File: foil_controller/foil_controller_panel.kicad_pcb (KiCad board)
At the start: 2 copper layers, 90 x 110 mm, 4 parts

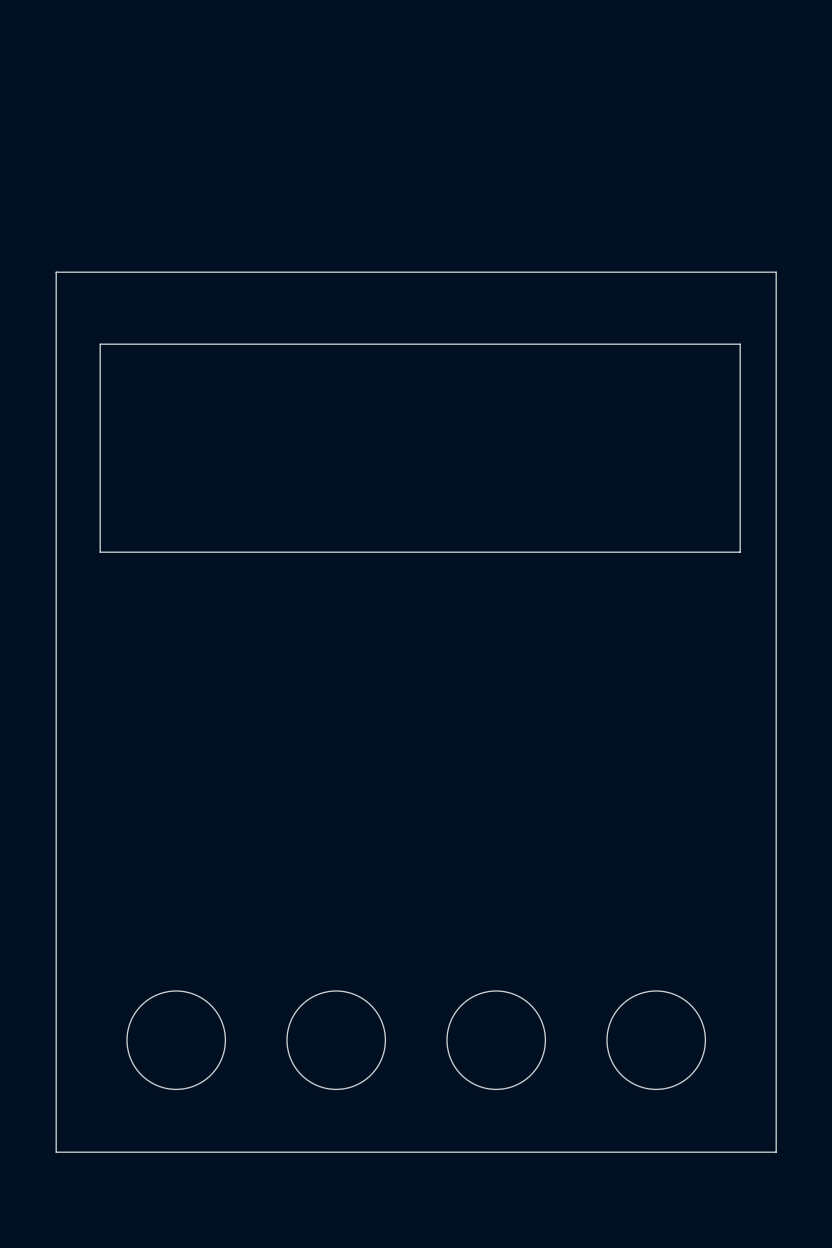
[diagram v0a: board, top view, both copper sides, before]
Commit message: controller v2 voor testvaart 1 mei
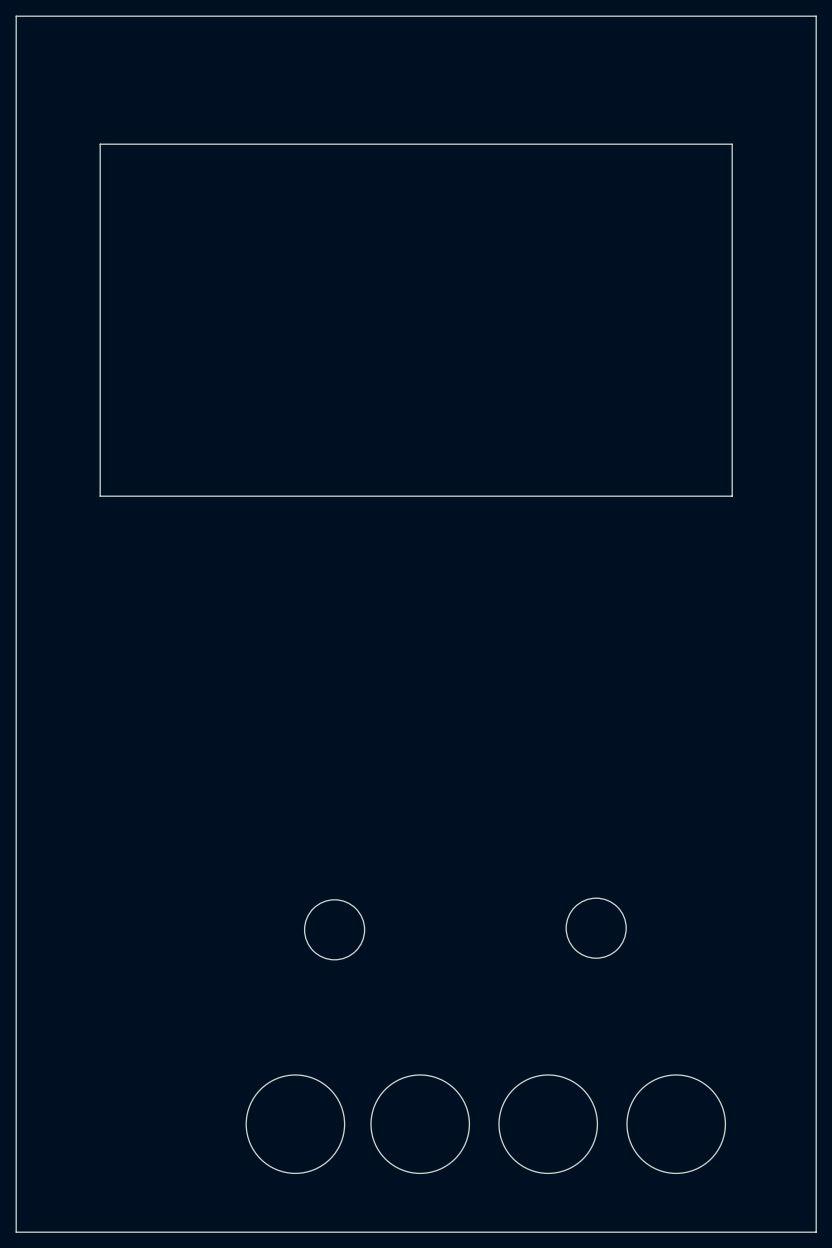
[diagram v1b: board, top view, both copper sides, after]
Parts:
- removed the H1 at (15.0, 96.0)
- removed the H1 at (35.0, 96.0)
- removed the H1 at (75.0, 96.0)
- removed the H1 at (55.0, 96.0)
- added H1: hole, MountingHole:MountingHole_3.2mm_M3_DIN965, F.Cu at (67.5, 82.0)
- added H1: hole, MountingHole:MountingHole_3.2mm_M3_DIN965, F.Cu at (34.8, 82.2)
- added H1: hole, MountingHole:MountingHole_3.2mm_M3_DIN965, F.Cu at (29.9, 106.5)
- added H1: hole, MountingHole:MountingHole_3.2mm_M3_DIN965, F.Cu at (45.5, 106.5)
- added H1: hole, MountingHole:MountingHole_3.2mm_M3_DIN965, F.Cu at (77.5, 106.5)
- added H1: hole, MountingHole:MountingHole_3.2mm_M3_DIN965, F.Cu at (61.5, 106.5)
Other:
- board size 90 x 110 mm -> 100 x 152 mm
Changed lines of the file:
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@@
     (tracks 0)
     (zones 0)
-    (modules 4)
+    (modules 6)
     (nets 1)
   )
@@
       (outputformat 1)
       (mirror false)
-      (drillshape 0)
+      (drillshape 1)
       (scaleselection 1)
-      (outputdirectory "out/"))
+      (outputdirectory ""))
   )
   (net 0 "")
@@
   )
   (module MountingHole:MountingHole_3.2mm_M3_DIN965 (layer F.Cu)
-    (at 15 96)
-    (descr hole)
-    (tags hole)
-    (attr virtual)
-    (fp_text reference H1 (at 0 -3.8) (layer F.SilkS) hide
-      (effects (font (size 1 1) (thickness 0.15)))
-    )
-    (fp_text value hole (at 0 3.8) (layer F.Fab) hide
-      (effects (font (size 1 1) (thickness 0.15)))
-    )
-    (fp_circle (center 0 0) (end 3.05 0) (layer F.CrtYd) (width 0.05))
-    (fp_circle (center 0 0) (end 2.8 0) (layer Cmts.User) (width 0.15))
-    (fp_text user %R (at 0.3 0) (layer F.Fab)
-      (effects (font (size 1 1) (thickness 0.15)))
-    )
-    (pad 1 np_thru_hole circle (at 0 0) (size 12.3 12.3) (drill 12.3) (layers *.Cu *.Mask))
-  )
-  (module MountingHole:MountingHole_3.2mm_M3_DIN965 (layer F.Cu)
-    (at 35 96)
-    (descr hole)
-    (tags hole)
-    (attr virtual)
-    (fp_text reference H1 (at 0 -3.8) (layer F.SilkS) hide
-      (effects (font (size 1 1) (thickness 0.15)))
-    )
-    (fp_text value hole (at 0 3.8) (layer F.Fab) hide
-      (effects (font (size 1 1) (thickness 0.15)))
-    )
-    (fp_circle (center 0 0) (end 3.05 0) (layer F.CrtYd) (width 0.05))
-    (fp_circle (center 0 0) (end 2.8 0) (layer Cmts.User) (width 0.15))
-    (fp_text user %R (at 0.3 0) (layer F.Fab)
-      (effects (font (size 1 1) (thickness 0.15)))
-    )
-    (pad 1 np_thru_hole circle (at 0 0) (size 12.3 12.3) (drill 12.3) (layers *.Cu *.Mask))
-  )
-  (module MountingHole:MountingHole_3.2mm_M3_DIN965 (layer F.Cu)
-    (at 75 96)
-    (descr hole)
-    (tags hole)
-    (attr virtual)
-    (fp_text reference H1 (at 0 -3.8) (layer F.SilkS) hide
-      (effects (font (size 1 1) (thickness 0.15)))
-    )
-    (fp_text value hole (at 0 3.8) (layer F.Fab) hide
-      (effects (font (size 1 1) (thickness 0.15)))
-    )
-    (fp_circle (center 0 0) (end 3.05 0) (layer F.CrtYd) (width 0.05))
-    (fp_circle (center 0 0) (end 2.8 0) (layer Cmts.User) (width 0.15))
-    (fp_text user %R (at 0.3 0) (layer F.Fab)
-      (effects (font (size 1 1) (thickness 0.15)))
-    )
-    (pad 1 np_thru_hole circle (at 0 0) (size 12.3 12.3) (drill 12.3) (layers *.Cu *.Mask))
-  )
-  (module MountingHole:MountingHole_3.2mm_M3_DIN965 (layer F.Cu)
-    (at 55 96)
-    (descr hole)
-    (tags hole)
-    (attr virtual)
-    (fp_text reference H1 (at 0 -3.8) (layer F.SilkS) hide
-      (effects (font (size 1 1) (thickness 0.15)))
-    )
-    (fp_text value hole (at 0 3.8) (layer F.Fab) hide
-      (effects (font (size 1 1) (thickness 0.15)))
-    )
-    (fp_circle (center 0 0) (end 3.05 0) (layer F.CrtYd) (width 0.05))
-    (fp_circle (center 0 0) (end 2.8 0) (layer Cmts.User) (width 0.15))
-    (fp_text user %R (at 0.3 0) (layer F.Fab)
-      (effects (font (size 1 1) (thickness 0.15)))
-    )
-    (pad 1 np_thru_hole circle (at 0 0) (size 12.3 12.3) (drill 12.3) (layers *.Cu *.Mask))
-  )
-  (gr_line (start 5.5 35) (end 85.5 35) (layer Edge.Cuts) (width 0.05))
-  (gr_line (start 5.5 9) (end 5.5 35) (layer Edge.Cuts) (width 0.05))
-  (gr_line (start 85.5 9) (end 5.5 9) (layer Edge.Cuts) (width 0.05))
-  (gr_line (start 85.5 35) (end 85.5 9) (layer Edge.Cuts) (width 0.05))
-  (gr_line (start 0 110) (end 0 0) (layer Edge.Cuts) (width 0.05))
-  (gr_line (start 90 110) (end 0 110) (layer Edge.Cuts) (width 0.05))
-  (gr_line (start 90 0) (end 90 110) (layer Edge.Cuts) (width 0.05))
-  (gr_line (start 0 0) (end 90 0) (layer Edge.Cuts) (width 0.05))
+    (at 67.5 82)
+    (descr hole)
+    (tags hole)
+    (attr virtual)
+    (fp_text reference H1 (at 0 -3.8) (layer F.SilkS) hide
+      (effects (font (size 1 1) (thickness 0.15)))
+    )
+    (fp_text value hole (at 0 3.8) (layer F.Fab) hide
+      (effects (font (size 1 1) (thickness 0.15)))
+    )
+    (fp_circle (center 0 0) (end 3.05 0) (layer F.CrtYd) (width 0.05))
+    (fp_circle (center 0 0) (end 2.8 0) (layer Cmts.User) (width 0.15))
+    (fp_text user %R (at 0.3 0) (layer F.Fab)
+      (effects (font (size 1 1) (thickness 0.15)))
+    )
+    (pad 1 np_thru_hole circle (at 0 0) (size 7.5 7.5) (drill 7.5) (layers *.Cu *.Mask))
+  )
+  (module MountingHole:MountingHole_3.2mm_M3_DIN965 (layer F.Cu)
+    (at 34.8 82.2)
+    (descr hole)
+    (tags hole)
+    (attr virtual)
+    (fp_text reference H1 (at 0 -3.8) (layer F.SilkS) hide
+      (effects (font (size 1 1) (thickness 0.15)))
+    )
+    (fp_text value hole (at 0 3.8) (layer F.Fab) hide
+      (effects (font (size 1 1) (thickness 0.15)))
+    )
+    (fp_circle (center 0 0) (end 3.05 0) (layer F.CrtYd) (width 0.05))
+    (fp_circle (center 0 0) (end 2.8 0) (layer Cmts.User) (width 0.15))
+    (fp_text user %R (at 0.3 0) (layer F.Fab)
+      (effects (font (size 1 1) (thickness 0.15)))
+    )
+    (pad 1 np_thru_hole circle (at 0 0) (size 7.5 7.5) (drill 7.5) (layers *.Cu *.Mask))
+  )
+  (module MountingHole:MountingHole_3.2mm_M3_DIN965 (layer F.Cu)
+    (at 29.9 106.5)
+    (descr hole)
+    (tags hole)
+    (attr virtual)
+    (fp_text reference H1 (at 0 -3.8) (layer F.SilkS) hide
+      (effects (font (size 1 1) (thickness 0.15)))
+    )
+    (fp_text value hole (at 0 3.8) (layer F.Fab) hide
+      (effects (font (size 1 1) (thickness 0.15)))
+    )
+    (fp_circle (center 0 0) (end 3.05 0) (layer F.CrtYd) (width 0.05))
+    (fp_circle (center 0 0) (end 2.8 0) (layer Cmts.User) (width 0.15))
+    (fp_text user %R (at 0.3 0) (layer F.Fab)
+      (effects (font (size 1 1) (thickness 0.15)))
+    )
+    (pad 1 np_thru_hole circle (at 0 0) (size 12.3 12.3) (drill 12.3) (layers *.Cu *.Mask))
+  )
+  (module MountingHole:MountingHole_3.2mm_M3_DIN965 (layer F.Cu)
+    (at 45.5 106.5)
+    (descr hole)
+    (tags hole)
+    (attr virtual)
+    (fp_text reference H1 (at 0 -3.8) (layer F.SilkS) hide
+      (effects (font (size 1 1) (thickness 0.15)))
+    )
+    (fp_text value hole (at 0 3.8) (layer F.Fab) hide
+      (effects (font (size 1 1) (thickness 0.15)))
+    )
+    (fp_circle (center 0 0) (end 3.05 0) (layer F.CrtYd) (width 0.05))
+    (fp_circle (center 0 0) (end 2.8 0) (layer Cmts.User) (width 0.15))
+    (fp_text user %R (at 0.3 0) (layer F.Fab)
+      (effects (font (size 1 1) (thickness 0.15)))
+    )
+    (pad 1 np_thru_hole circle (at 0 0) (size 12.3 12.3) (drill 12.3) (layers *.Cu *.Mask))
+  )
+  (module MountingHole:MountingHole_3.2mm_M3_DIN965 (layer F.Cu)
+    (at 77.5 106.5)
+    (descr hole)
+    (tags hole)
+    (attr virtual)
+    (fp_text reference H1 (at 0 -3.8) (layer F.SilkS) hide
+      (effects (font (size 1 1) (thickness 0.15)))
+    )
+    (fp_text value hole (at 0 3.8) (layer F.Fab) hide
+      (effects (font (size 1 1) (thickness 0.15)))
+    )
+    (fp_circle (center 0 0) (end 3.05 0) (layer F.CrtYd) (width 0.05))
+    (fp_circle (center 0 0) (end 2.8 0) (layer Cmts.User) (width 0.15))
+    (fp_text user %R (at 0.3 0) (layer F.Fab)
+      (effects (font (size 1 1) (thickness 0.15)))
+    )
+    (pad 1 np_thru_hole circle (at 0 0) (size 12.3 12.3) (drill 12.3) (layers *.Cu *.Mask))
+  )
+  (module MountingHole:MountingHole_3.2mm_M3_DIN965 (layer F.Cu)
+    (at 61.5 106.5)
+    (descr hole)
+    (tags hole)
+    (attr virtual)
+    (fp_text reference H1 (at 0 -3.8) (layer F.SilkS) hide
+      (effects (font (size 1 1) (thickness 0.15)))
+    )
+    (fp_text value hole (at 0 3.8) (layer F.Fab) hide
+      (effects (font (size 1 1) (thickness 0.15)))
+    )
+    (fp_circle (center 0 0) (end 3.05 0) (layer F.CrtYd) (width 0.05))
+    (fp_circle (center 0 0) (end 2.8 0) (layer Cmts.User) (width 0.15))
+    (fp_text user %R (at 0.3 0) (layer F.Fab)
+      (effects (font (size 1 1) (thickness 0.15)))
+    )
+    (pad 1 np_thru_hole circle (at 0 0) (size 12.3 12.3) (drill 12.3) (layers *.Cu *.Mask))
+  )
+  (gr_line (start 5.5 28) (end 84.5 28) (layer Edge.Cuts) (width 0.05))
+  (gr_line (start 5.5 -16) (end 5.5 28) (layer Edge.Cuts) (width 0.05))
+  (gr_line (start 84.5 -16) (end 5.5 -16) (layer Edge.Cuts) (width 0.05))
+  (gr_line (start 84.5 28) (end 84.5 -16) (layer Edge.Cuts) (width 0.05))
+  (gr_line (start -5 120) (end -5 -32) (layer Edge.Cuts) (width 0.05))
+  (gr_line (start 95 120) (end -5 120) (layer Edge.Cuts) (width 0.05))
+  (gr_line (start 95 -32) (end 95 120) (layer Edge.Cuts) (width 0.05))
+  (gr_line (start -5 -32) (end 95 -32) (layer Edge.Cuts) (width 0.05))
 )
